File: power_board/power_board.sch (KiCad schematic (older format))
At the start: 79 parts, among them J1 PROG, J10 M4, J11 5V_1, J12 M5, J13 M6, J14 M7, J15 FAN, J16 Screw_Terminal_01x02, J17 MB_interface, J18 Conn_01x02_Female, J19 12V_1, J2 M1, J20 12V_2, J21 12V_3, J22 12V_4, J23 48V_1, J24 48V_2, J25 48V_3, J26 48V_4, J27 Screw_Terminal_01x02, J3 M2, J4 Conn_01x02_Female, J5 Conn_01x02_Female, J6 Conn_01x01_Male, J7 Conn_01x01_Male, J8 Screw_Terminal_01x02, J9 M3, Q1 2N3906, SW1 SW_Push, U1 ACS758xCB-050B-PFF, U10 MAX31855KASA, U2 ACS758xCB-050B-PFF, U3 MCP2515-EST, U4 MAX31855KASA, U5 MCP2551-I-SN, U6 BTS50085-1TMA, U7 ATmega328P-AU, U8 BTS50085-1TMA, U9 LM2596S-5, Y1 20Mhz, Y2 16Mhz

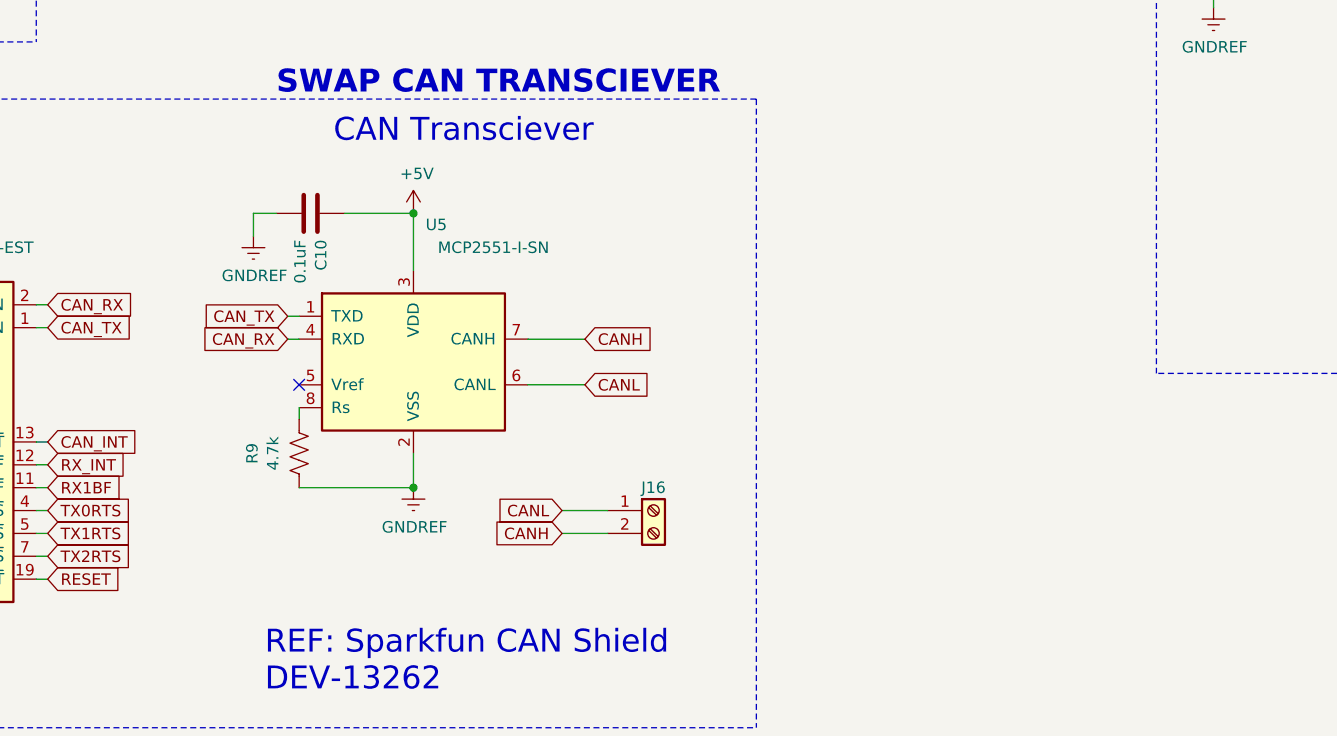
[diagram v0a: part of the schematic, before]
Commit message: Added 3d models, finished design
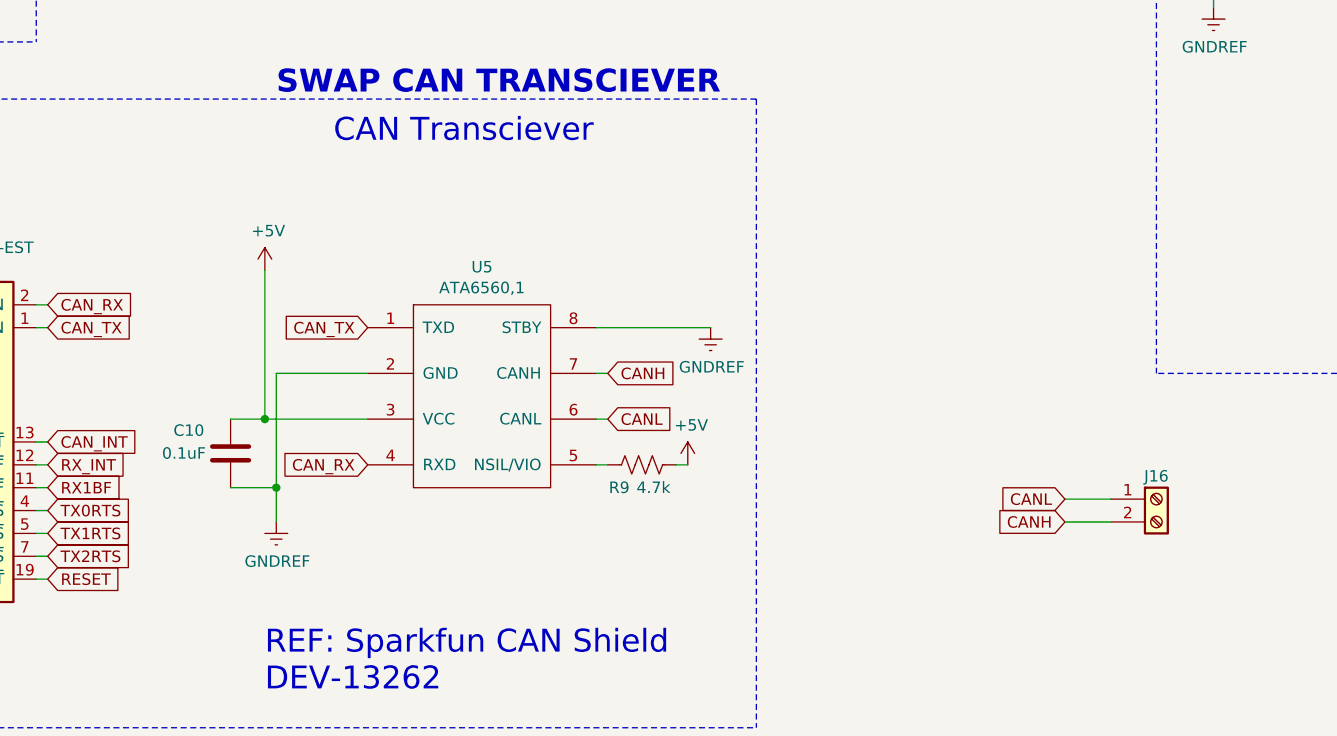
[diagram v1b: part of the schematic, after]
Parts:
- removed U5: MCP2551-I-SN, Package_SO:SOIC-8_3.9x4.9mm_P1.27mm, symbol Interface_CAN_LIN:MCP2551-I-SN
- added U5: ATA6560,1, Package_SO:SOIC-8_3.9x4.9mm_P1.27mm, symbol URT_cache:ATA6560,1
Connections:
- net +5V: now also R9.2, U5.3 (VCC)
- net CANH: now also U5.7 (CANH)
- net CANL: now also U5.6 (CANL)
- net CAN_RX: now also U5.4 (RXD)
- net CAN_TX: now also U5.1 (TXD)
- net GNDREF: now also U5.2 (GND), U5.8 (STBY); no longer R9.1
- new net: R9.1, U5.5 (NSIL/VIO)
- no-connect marks 13 -> 12
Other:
- moved on the sheet: C10, J16
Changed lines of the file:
@@
-$EndComp
-$Comp
-L Interface_CAN_LIN:MCP2551-I-SN U5
-U 1 1 5BA69EE0
-P 9850 8200
-F 0 "U5" H 9950 8800 50  0000 C CNN
-F 1 "MCP2551-I-SN" H 10200 8700 50  0000 C CNN
-F 2 "Package_SO:SOIC-8_3.9x4.9mm_P1.27mm" H 9850 7700 50  0001 C CIN
-F 3 "http://ww1.microchip.com/downloads/en/devicedoc/21667d.pdf" H 9850 8200 50  0001 C CNN
-	1    9850 8200
-	1    0    0    -1
-$EndComp
-Text GLabel 9300 8000 0    50   Input ~ 0
-CAN_TX
-Text GLabel 9300 8100 0    50   Input ~ 0
-CAN_RX
-$Comp
-L power:+5V #PWR0143
-U 1 1 5BA77637
-P 9850 7550
-F 0 "#PWR0143" H 9850 7400 50  0001 C CNN
-F 1 "+5V" H 9865 7723 50  0000 C CNN
-F 2 "" H 9850 7550 50  0001 C CNN
-F 3 "" H 9850 7550 50  0001 C CNN
-	1    9850 7550
-	1    0    0    -1
-$EndComp
-$Comp
-L power:GNDREF #PWR0144
-U 1 1 5BA77D6B
-P 9850 8750
-F 0 "#PWR0144" H 9850 8500 50  0001 C CNN
-F 1 "GNDREF" H 9855 8577 50  0000 C CNN
-F 2 "" H 9850 8750 50  0001 C CNN
-F 3 "" H 9850 8750 50  0001 C CNN
-	1    9850 8750
-	1    0    0    -1
 $EndComp
 $Comp
 L Device:C C10
 U 1 1 5BA784CE
-P 9400 7550
-F 0 "C10" H 9515 7596 50  0000 L CNN
-F 1 "0.1uF" H 9515 7505 50  0000 L CNN
-F 2 "Capacitor_SMD:C_0603_1608Metric" H 9438 7400 50  0001 C CNN
-F 3 "~" H 9400 7550 50  0001 C CNN
-	1    9400 7550
-	0    1    1    0
-$EndComp
-$Comp
-L power:GNDREF #PWR0145
-U 1 1 5BA788D6
-P 9150 7650
-F 0 "#PWR0145" H 9150 7400 50  0001 C CNN
-F 1 "GNDREF" H 9155 7477 50  0000 C CNN
-F 2 "" H 9150 7650 50  0001 C CNN
-F 3 "" H 9150 7650 50  0001 C CNN
-	1    9150 7650
-	1    0    0    -1
-$EndComp
-Wire Wire Line
-	9850 7550 9850 7800
-Wire Wire Line
-	9550 7550 9850 7550
-Connection ~ 9850 7550
-Wire Wire Line
-	9250 7550 9150 7550
-Wire Wire Line
-	9150 7550 9150 7650
-Wire Wire Line
-	9300 8000 9350 8000
-Wire Wire Line
-	9300 8100 9350 8100
+P 9050 8600
+F 0 "C10" H 8800 8700 50  0000 L CNN
+F 1 "0.1uF" H 8750 8600 50  0000 L CNN
+F 2 "Capacitor_SMD:C_0603_1608Metric" H 9088 8450 50  0001 C CNN
+F 3 "~" H 9050 8600 50  0001 C CNN
+	1    9050 8600
+	1    0    0    -1
+$EndComp
 $Comp
 L power:+5V #PWR0146
@@
 Wire Wire Line
 	8200 8050 8250 8050
-$Comp
-L Device:R_US R9
-U 1 1 5BB7FA96
-P 9350 8600
-F 0 "R9" V 9555 8600 50  0000 C CNN
-F 1 "4.7k" V 9464 8600 50  0000 C CNN
-F 2 "Resistor_SMD:R_0603_1608Metric" V 9390 8590 50  0001 C CNN
-F 3 "~" H 9350 8600 50  0001 C CNN
-	1    9350 8600
-	-1   0    0    1
-$EndComp
-Wire Wire Line
-	9350 8400 9350 8450
-Wire Wire Line
-	9350 8750 9850 8750
-Wire Wire Line
-	9850 8600 9850 8750
-Connection ~ 9850 8750
-Text GLabel 10600 8100 2    50   Input ~ 0
-CANH
-Text GLabel 10600 8300 2    50   Input ~ 0
-CANL
 Text GLabel 8250 8550 2    50   Input ~ 0
 CAN_INT
@@
 Text Notes 2150 3500 0    100  ~ 0
 Power Regulation
-Wire Wire Line
-	10350 8300 10600 8300
-Wire Wire Line
-	10350 8100 10600 8100
 Text Notes 8800 6400 0    100  ~ 20
 VERIFY PIN ORDER!!!\n\n
@@
 NoConn ~ 3950 5900
 NoConn ~ 3950 4650
-NoConn ~ 9350 8300
 NoConn ~ 15050 7400
 NoConn ~ 15050 5000
@@
 L Connector:Screw_Terminal_01x02 J16
 U 1 1 5BEFA5C2
-P 10900 8850
-F 0 "J16" H 10900 8950 50  0000 C CNN
-F 1 "Screw_Terminal_01x02" H 10900 9400 50  0001 C CNN
-F 2 "TerminalBlock:TerminalBlock_bornier-2_P5.08mm" H 10900 8850 50  0001 C CNN
-F 3 "~" H 10900 8850 50  0001 C CNN
-	1    10900 8850
-	1    0    0    -1
-$EndComp
-Text GLabel 10500 8950 0    50   Input ~ 0
+P 13100 8800
+F 0 "J16" H 13100 8900 50  0000 C CNN
+F 1 "Screw_Terminal_01x02" H 13100 9350 50  0001 C CNN
+F 2 "TerminalBlock:TerminalBlock_bornier-2_P5.08mm" H 13100 8800 50  0001 C CNN
+F 3 "~" H 13100 8800 50  0001 C CNN
+	1    13100 8800
+	1    0    0    -1
+$EndComp
+Text GLabel 12700 8900 0    50   Input ~ 0
 CANH
-Text GLabel 10500 8850 0    50   Input ~ 0
+Text GLabel 12700 8800 0    50   Input ~ 0
 CANL
 $Comp
@@
 	13400 2950 13550 2950
 Wire Wire Line
-	10500 8850 10700 8850
-Wire Wire Line
-	10500 8950 10700 8950
+	12700 8800 12900 8800
+Wire Wire Line
+	12700 8900 12900 8900
 $Comp
 L power:+5V #PWR0159
@@
 Wire Wire Line
 	4550 8550 4550 8750
+$Comp
+L URT_cache:ATA6560,1 U5
+U 1 1 5BCC7310
+P 10150 8350
+F 0 "U5" H 10150 8915 50  0000 C CNN
+F 1 "ATA6560,1" H 10150 8824 50  0000 C CNN
+F 2 "Package_SO:SOIC-8_3.9x4.9mm_P1.27mm" H 10150 8850 50  0001 C CNN
+F 3 "" H 10150 8850 50  0001 C CNN
+	1    10150 8350
+	1    0    0    -1
+$EndComp
+$Comp
+L power:GNDREF #PWR0143
+U 1 1 5BD211AA
+P 9250 8900
+F 0 "#PWR0143" H 9250 8650 50  0001 C CNN
+F 1 "GNDREF" H 9255 8727 50  0000 C CNN
+F 2 "" H 9250 8900 50  0001 C CNN
+F 3 "" H 9250 8900 50  0001 C CNN
+	1    9250 8900
+	1    0    0    -1
+$EndComp
+Text GLabel 9650 8650 0    50   Input ~ 0
+CAN_RX
+Text GLabel 9650 8050 0    50   Input ~ 0
+CAN_TX
+$Comp
+L power:+5V #PWR0144
+U 1 1 5BD3FC89
+P 9200 7800
+F 0 "#PWR0144" H 9200 7650 50  0001 C CNN
+F 1 "+5V" H 9215 7973 50  0000 C CNN
+F 2 "" H 9200 7800 50  0001 C CNN
+F 3 "" H 9200 7800 50  0001 C CNN
+	1    9200 7800
+	1    0    0    -1
+$EndComp
+Wire Wire Line
+	9200 7800 9200 8450
+Text GLabel 10700 8450 2    50   Input ~ 0
+CANL
+Text GLabel 10700 8250 2    50   Input ~ 0
+CANH
+Wire Wire Line
+	10650 8250 10700 8250
+Wire Wire Line
+	10650 8450 10700 8450
+Wire Wire Line
+	9250 8250 9250 8750
+Wire Wire Line
+	9200 8450 9650 8450
+Wire Wire Line
+	9250 8250 9650 8250
+Wire Wire Line
+	9050 8450 9200 8450
+Connection ~ 9200 8450
+Wire Wire Line
+	9050 8750 9250 8750
+Connection ~ 9250 8750
+Wire Wire Line
+	9250 8750 9250 8900
+$Comp
+L Device:R_US R9
+U 1 1 5BE74A3F
+P 10850 8650
+F 0 "R9" V 10750 8750 50  0000 C CNN
+F 1 "4.7k" V 10750 8600 50  0000 C CNN
+F 2 "Resistor_SMD:R_0603_1608Metric" V 10890 8640 50  0001 C CNN
+F 3 "~" H 10850 8650 50  0001 C CNN
+	1    10850 8650
+	0    -1   -1   0
+$EndComp
+Wire Wire Line
+	10650 8650 10700 8650
+$Comp
+L power:+5V #PWR0145
+U 1 1 5BE94E58
+P 11050 8650
+F 0 "#PWR0145" H 11050 8500 50  0001 C CNN
+F 1 "+5V" H 11065 8823 50  0000 C CNN
+F 2 "" H 11050 8650 50  0001 C CNN
+F 3 "" H 11050 8650 50  0001 C CNN
+	1    11050 8650
+	1    0    0    -1
+$EndComp
+Wire Wire Line
+	11000 8650 11050 8650
+$Comp
+L power:GNDREF #PWR0152
+U 1 1 5BEB4CDE
+P 11150 8050
+F 0 "#PWR0152" H 11150 7800 50  0001 C CNN
+F 1 "GNDREF" H 11155 7877 50  0000 C CNN
+F 2 "" H 11150 8050 50  0001 C CNN
+F 3 "" H 11150 8050 50  0001 C CNN
+	1    11150 8050
+	1    0    0    -1
+$EndComp
+Wire Wire Line
+	10650 8050 11150 8050
 $EndSCHEMATC

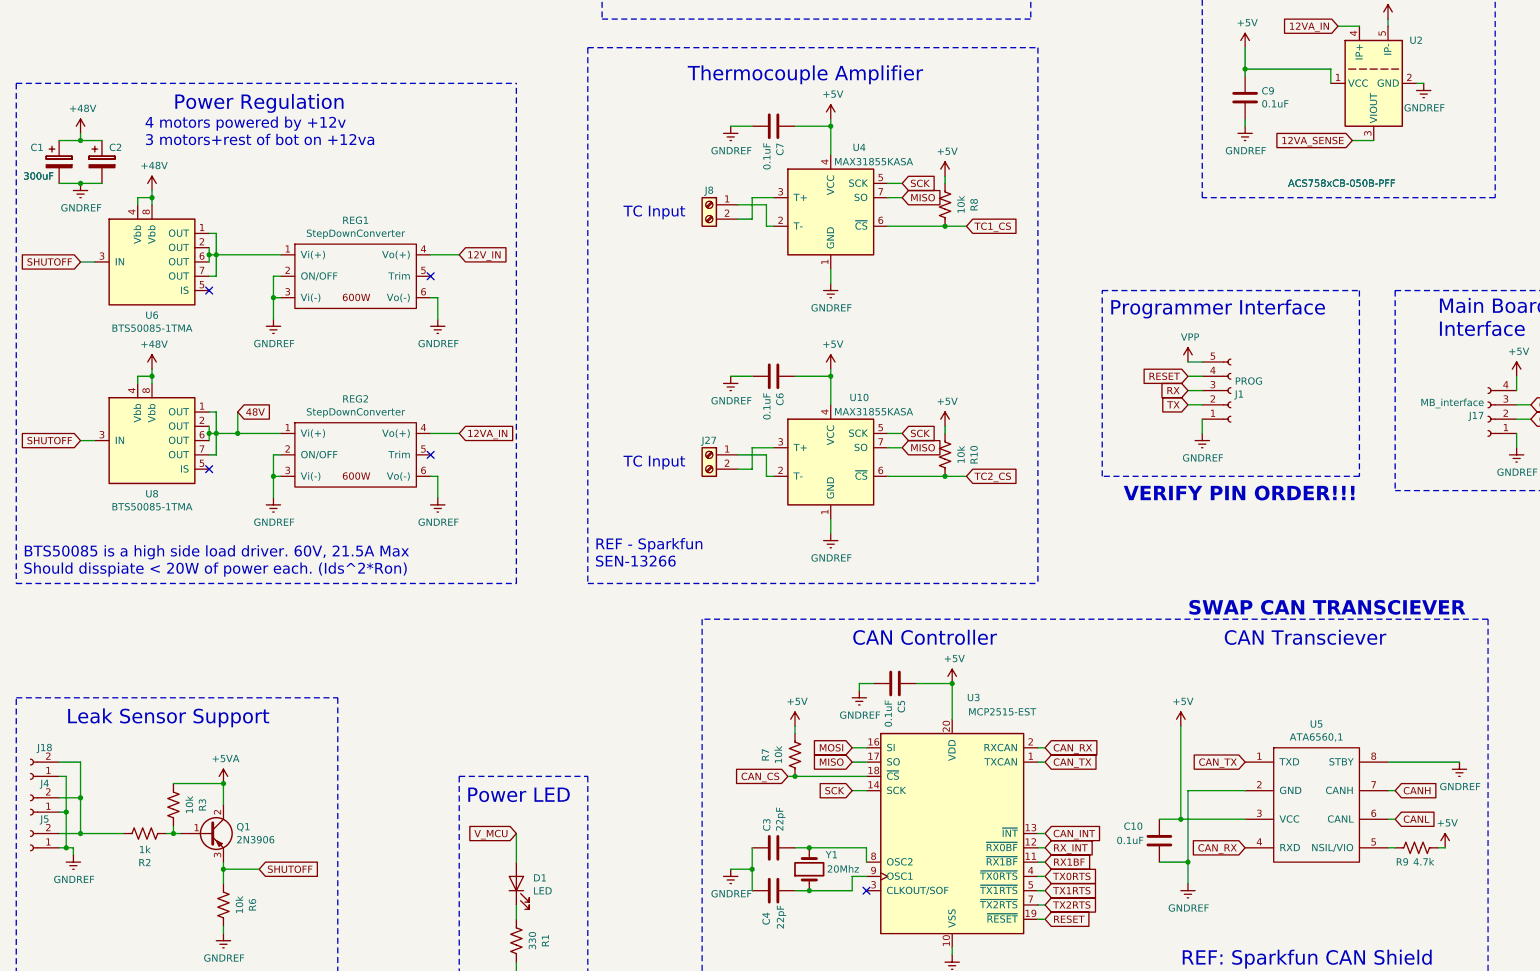
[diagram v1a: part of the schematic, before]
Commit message: capacitor updates
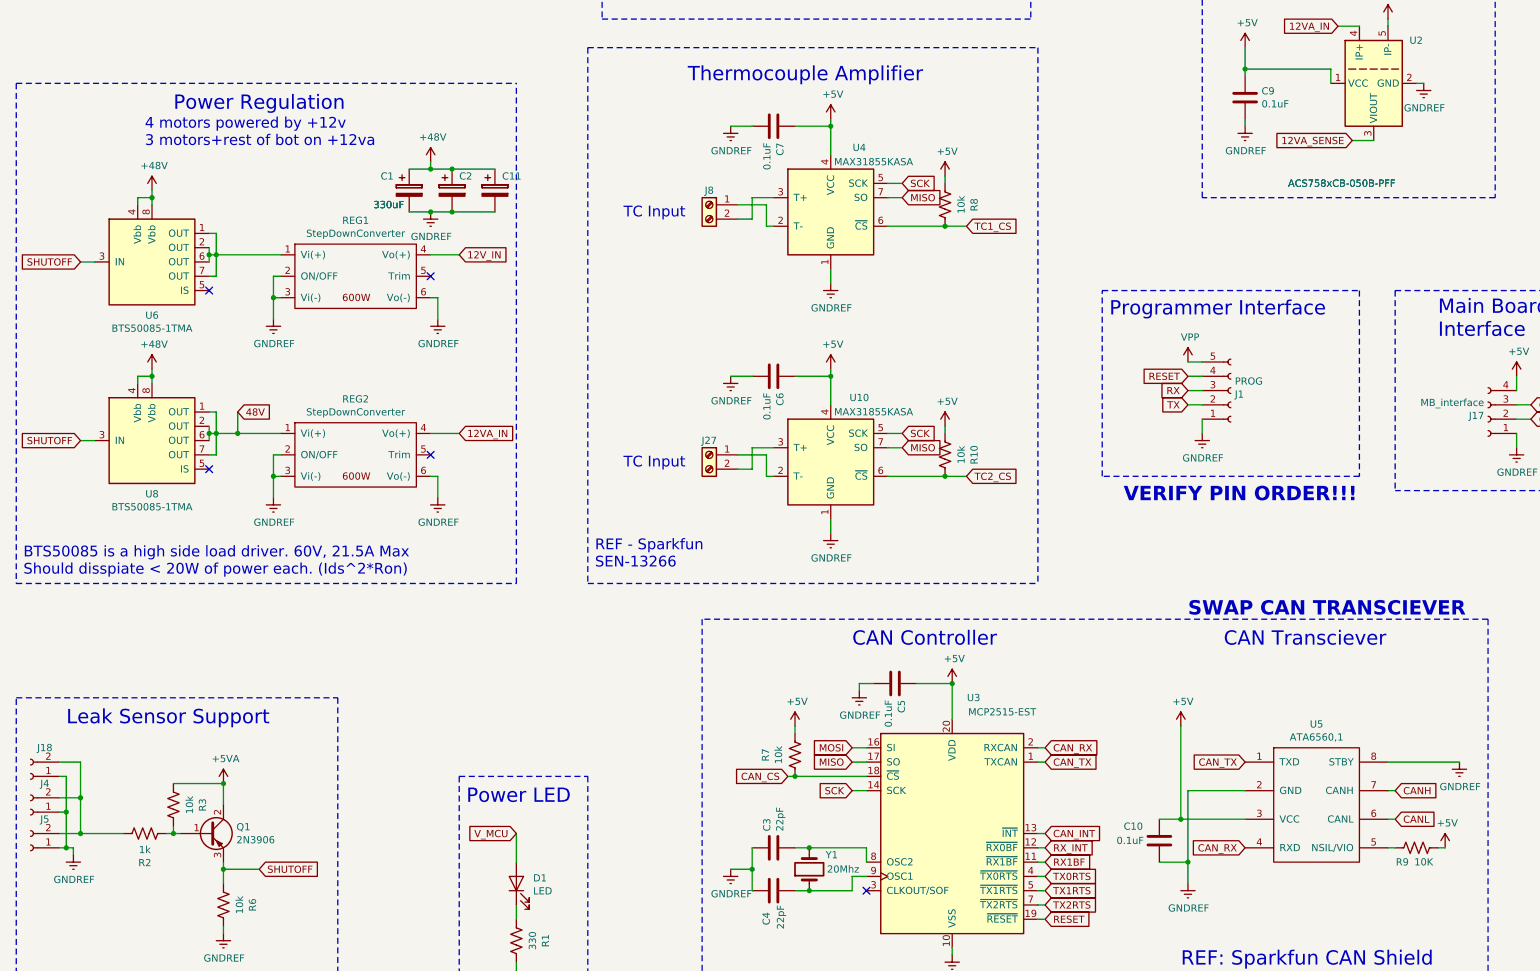
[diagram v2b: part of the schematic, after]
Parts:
- added C11: 330uF, Capacitor_THT:CP_Radial_D10.0mm_P5.00mm, symbol Device:CP
- C1, C2: value 300uF -> 330uF; footprint Capacitor_THT:CP_Radial_D10.0mm_P7.50mm -> Capacitor_THT:CP_Radial_D10.0mm_P5.00mm
- R9: value 4.7k -> 10K
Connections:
- net +48V: now also C11.1
- net GNDREF: now also C11.2
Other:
- moved on the sheet: C1, C2
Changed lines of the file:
@@
 L Device:CP C1
 U 1 1 5BA44640
-P 1350 3850
-F 0 "C1" H 1150 3950 50  0000 L CNN
-F 1 "300uF" H 1100 3750 50  0000 L CNN
-F 2 "Capacitor_THT:CP_Radial_D10.0mm_P7.50mm" H 1388 3700 50  0001 C CNN
-F 3 "~" H 1350 3850 50  0001 C CNN
-	1    1350 3850
+P 3800 4050
+F 0 "C1" H 3600 4150 50  0000 L CNN
+F 1 "330uF" H 3550 3950 50  0000 L CNN
+F 2 "Capacitor_THT:CP_Radial_D10.0mm_P5.00mm" H 3838 3900 50  0001 C CNN
+F 3 "~" H 3800 4050 50  0001 C CNN
+	1    3800 4050
 	1    0    0    -1
 $EndComp
@@
 L Device:CP C2
 U 1 1 5BA446DC
-P 1650 3850
-F 0 "C2" H 1700 3950 50  0000 L CNN
-F 1 "300uF" H 1100 3750 50  0000 L CNN
-F 2 "Capacitor_THT:CP_Radial_D10.0mm_P7.50mm" H 1688 3700 50  0001 C CNN
-F 3 "~" H 1650 3850 50  0001 C CNN
-	1    1650 3850
+P 4100 4050
+F 0 "C2" H 4150 4150 50  0000 L CNN
+F 1 "330uF" H 3550 3950 50  0000 L CNN
+F 2 "Capacitor_THT:CP_Radial_D10.0mm_P5.00mm" H 4138 3900 50  0001 C CNN
+F 3 "~" H 4100 4050 50  0001 C CNN
+	1    4100 4050
 	1    0    0    -1
 $EndComp
@@
 L power:GNDREF #PWR0101
 U 1 1 5BABAFE5
-P 1500 4000
-F 0 "#PWR0101" H 1500 3750 50  0001 C CNN
-F 1 "GNDREF" H 1505 3827 50  0000 C CNN
-F 2 "" H 1500 4000 50  0001 C CNN
-F 3 "" H 1500 4000 50  0001 C CNN
-	1    1500 4000
+P 3950 4200
+F 0 "#PWR0101" H 3950 3950 50  0001 C CNN
+F 1 "GNDREF" H 3955 4027 50  0000 C CNN
+F 2 "" H 3950 4200 50  0001 C CNN
+F 3 "" H 3950 4200 50  0001 C CNN
+	1    3950 4200
 	1    0    0    -1
 $EndComp
@@
 	2450 4500 2900 4500
 Wire Wire Line
-	1650 4000 1500 4000
-Wire Wire Line
-	1350 4000 1500 4000
-Connection ~ 1500 4000
-Wire Wire Line
-	1650 3700 1500 3700
+	4100 4200 3950 4200
+Wire Wire Line
+	3800 4200 3950 4200
+Connection ~ 3950 4200
+Wire Wire Line
+	4100 3900 3950 3900
 $Comp
 L power:+48V #PWR0161
 U 1 1 5BD4F164
-P 1500 3650
-F 0 "#PWR0161" H 1500 3500 50  0001 C CNN
-F 1 "+48V" H 1515 3823 50  0000 C CNN
-F 2 "" H 1500 3650 50  0001 C CNN
-F 3 "" H 1500 3650 50  0001 C CNN
-	1    1500 3650
-	1    0    0    -1
-$EndComp
-Wire Wire Line
-	1500 3650 1500 3700
-Connection ~ 1500 3700
-Wire Wire Line
-	1500 3700 1350 3700
+P 3950 3850
+F 0 "#PWR0161" H 3950 3700 50  0001 C CNN
+F 1 "+48V" H 3965 4023 50  0000 C CNN
+F 2 "" H 3950 3850 50  0001 C CNN
+F 3 "" H 3950 3850 50  0001 C CNN
+	1    3950 3850
+	1    0    0    -1
+$EndComp
+Wire Wire Line
+	3950 3850 3950 3900
+Connection ~ 3950 3900
+Wire Wire Line
+	3950 3900 3800 3900
 $Comp
 L power:GNDREF #PWR0162
@@
 P 10850 8650
 F 0 "R9" V 10750 8750 50  0000 C CNN
-F 1 "4.7k" V 10750 8600 50  0000 C CNN
+F 1 "10K" V 10750 8600 50  0000 C CNN
 F 2 "Resistor_SMD:R_0603_1608Metric" V 10890 8640 50  0001 C CNN
 F 3 "~" H 10850 8650 50  0001 C CNN
@@
 Wire Wire Line
 	10650 8050 11150 8050
+$Comp
+L Device:CP C11
+U 1 1 5BCFC50C
+P 4400 4050
+F 0 "C11" H 4450 4150 50  0000 L CNN
+F 1 "330uF" H 3550 3950 50  0000 L CNN
+F 2 "Capacitor_THT:CP_Radial_D10.0mm_P5.00mm" H 4438 3900 50  0001 C CNN
+F 3 "~" H 4400 4050 50  0001 C CNN
+	1    4400 4050
+	1    0    0    -1
+$EndComp
+Wire Wire Line
+	4100 3900 4400 3900
+Connection ~ 4100 3900
+Wire Wire Line
+	4100 4200 4400 4200
+Connection ~ 4100 4200
 $EndSCHEMATC
